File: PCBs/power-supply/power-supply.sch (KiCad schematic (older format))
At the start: 52 parts, among them J1 250V-A, J10 0V, J11 +310V-L, J12 0V, J13 +42V, J14 +42V, J15 0V, J16 0V, J17 +38V, J18 +38V, J19 0V, J2 250V-B, J20 0V, J21 -38V, J22 -38V, J3 30V-A, J4 30V-B, J5 28V-A, J6 28V-B, J7 28V-C, J8 28V-D, J9 +310V-R, U3 TL783

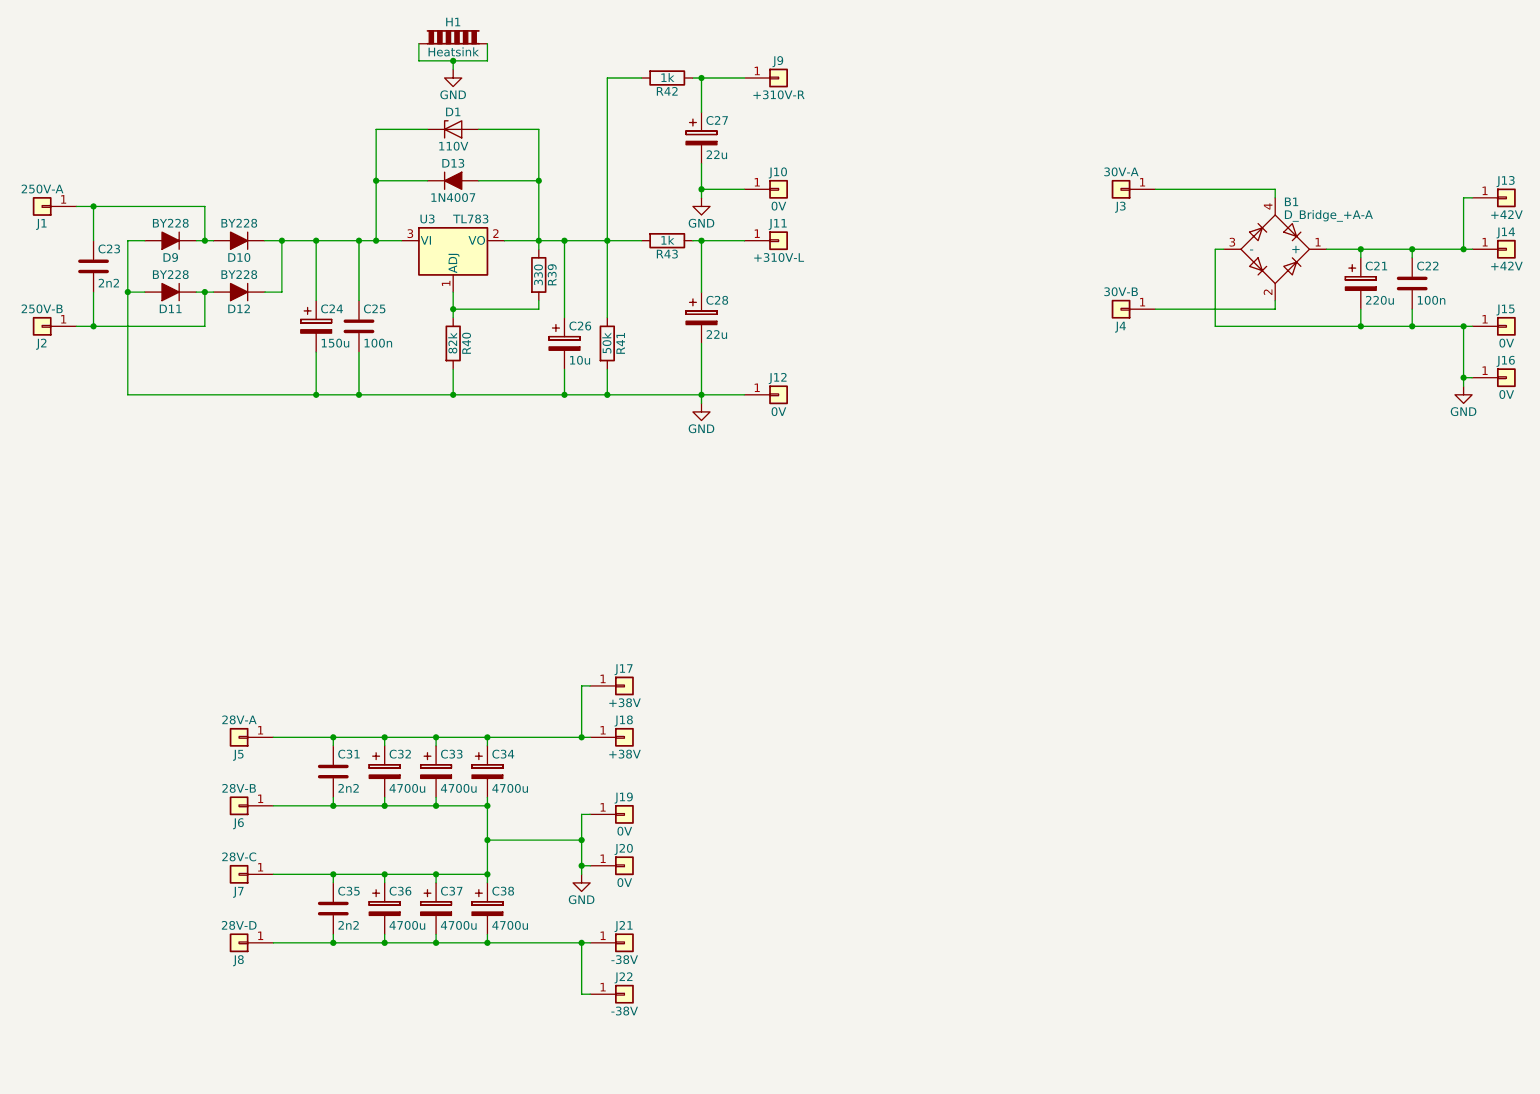
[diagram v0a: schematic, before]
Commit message: Small change.
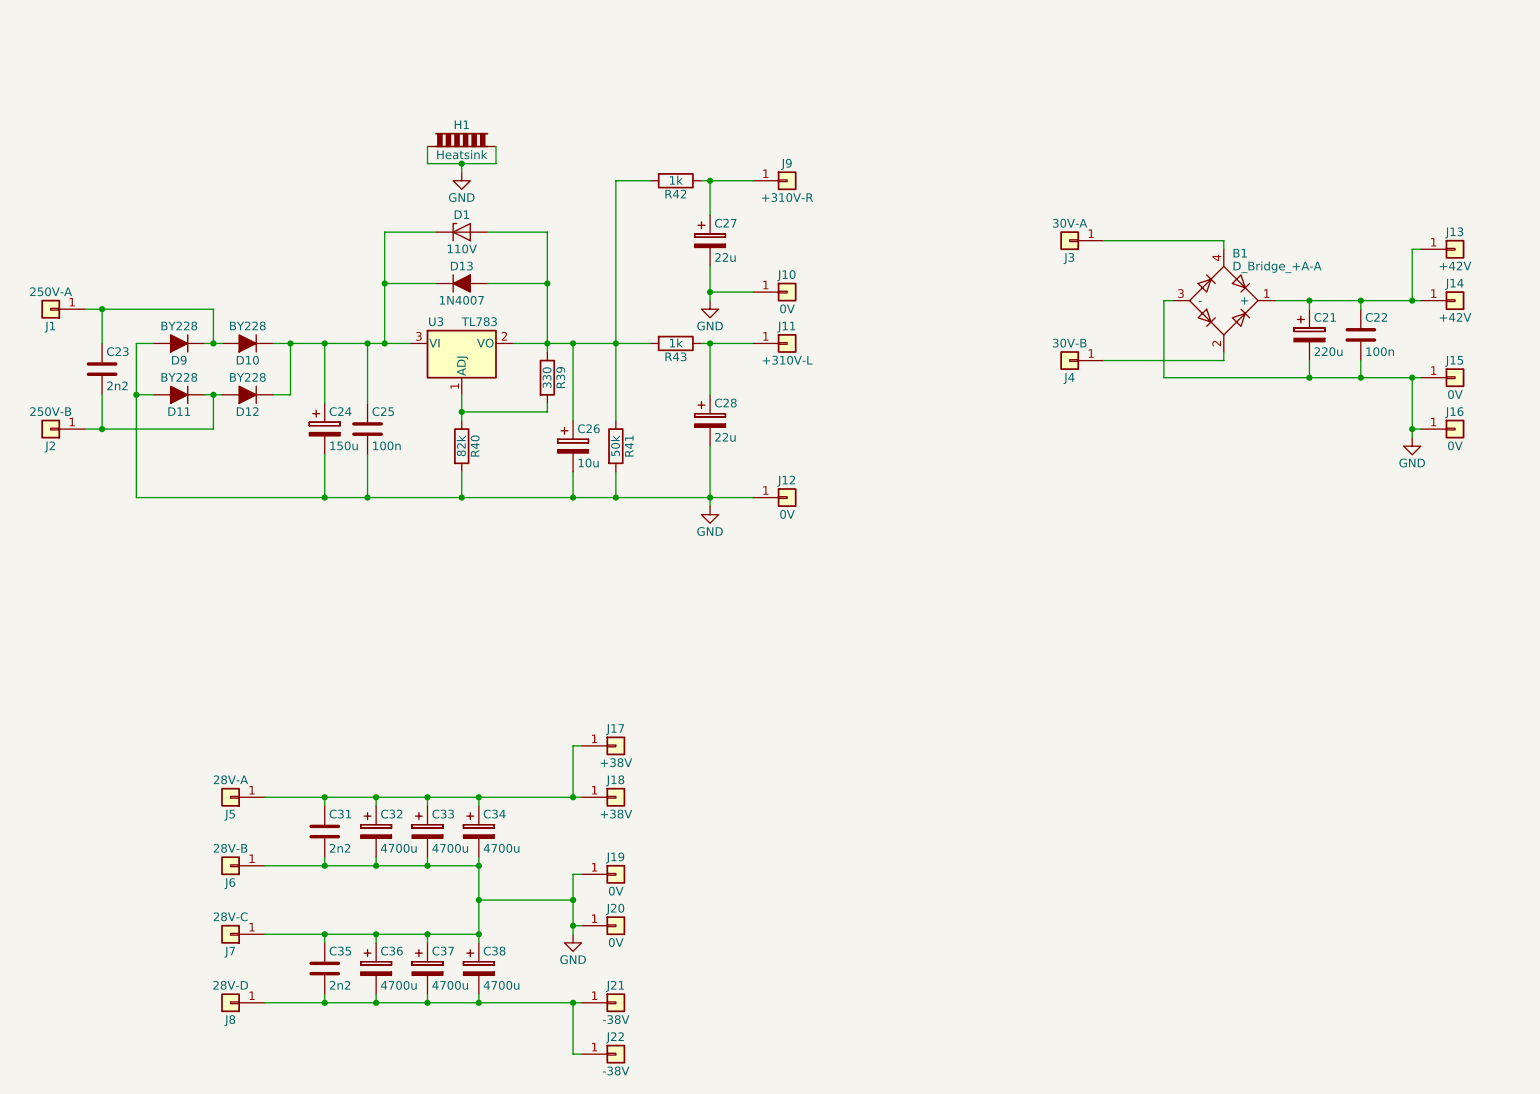
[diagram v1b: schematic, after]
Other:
- moved on the sheet: B1, C21, C22, C23, C24, C25, C26, C27, C28, C31, C32, C33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
